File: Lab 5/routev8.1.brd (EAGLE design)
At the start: 100 x 80 mm, 48 parts, among them J1 FTDI_DEVICE, M1 WIRELESS-NRF24L01, U2 GY-521MPU6050, U3 ATMEGA328P_TQFP

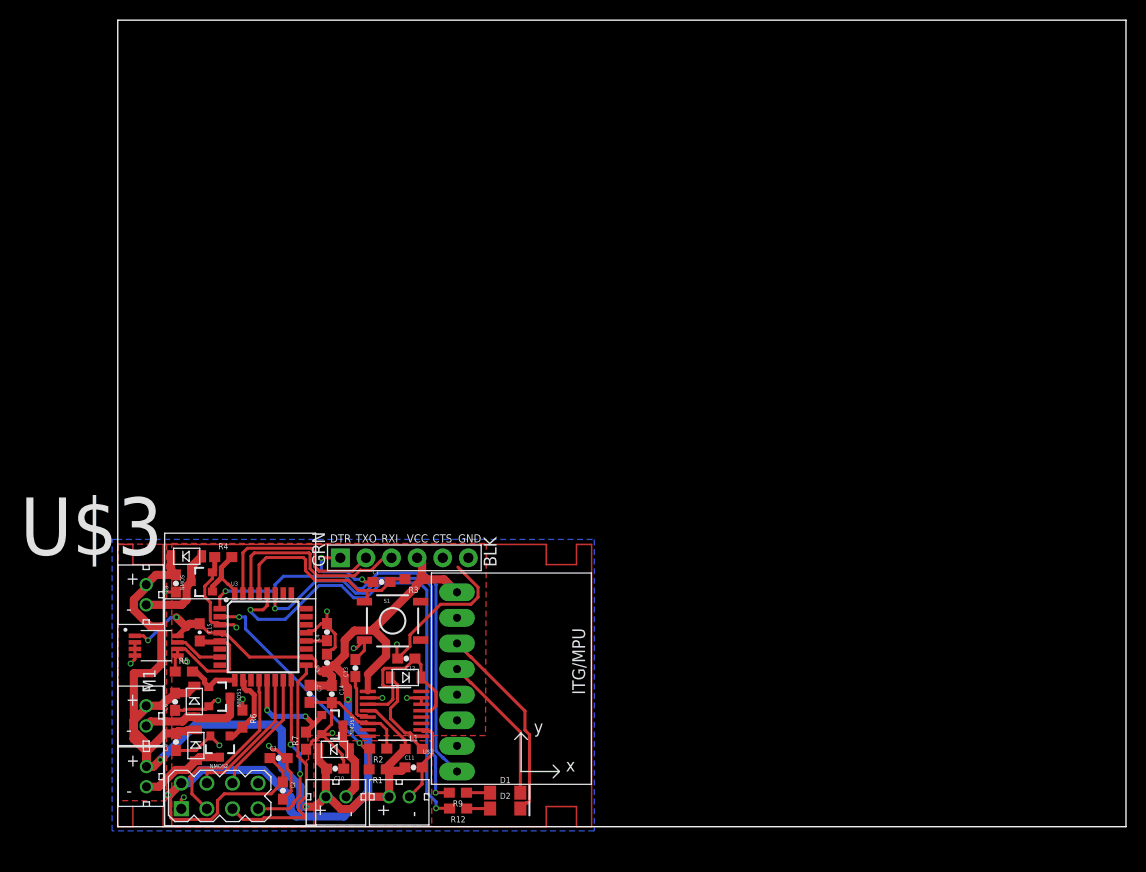
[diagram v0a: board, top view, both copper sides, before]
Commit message: We need a redesign guys
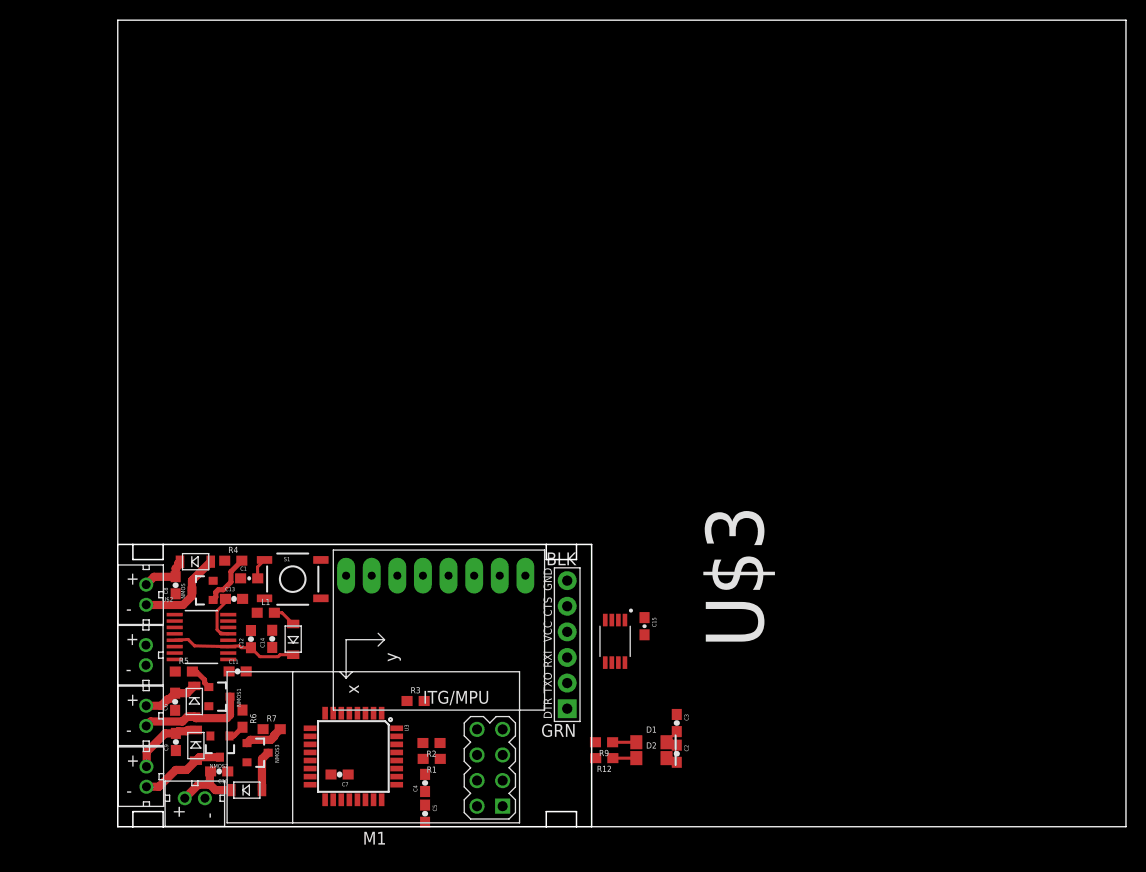
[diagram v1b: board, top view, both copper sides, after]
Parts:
- removed J1: FTDI_DEVICE, quad:FTDI_DEVICE_SIDE
- added J2: FTDI_DEVICE, quad:FTDI_DEVICE_SIDE
- C1: device SparkFun-Passives:0603-CAP -> SparkFun-Capacitors:0603-CAP
- R3: value 1k -> 10k
- moved U$3 45.5 mm to (49.3, 18.4), turned to 270 degrees
- moved C15 44.1 mm to (52.2, 19.9)
- moved C3 39.6 mm to (55.4, 10.3), turned to 270 degrees
- moved C2 39.2 mm to (55.4, 7.24)
- moved MOTOR3 23.5 mm to (2.79, 17.0), turned to 0 degrees
- moved U$2 20.6 mm to (8.30, 18.8), turned to 0 degrees
- moved U$1 20.3 mm to (7.65, 2.83)
- moved L1 19.9 mm to (14.7, 21.2)
- moved C11 19.9 mm to (11.9, 15.4)
- moved C4 17.8 mm to (30.5, 4.34)
- moved C5 17.8 mm to (30.5, 1.30), turned to 270 degrees
- moved C12 15.5 mm to (13.2, 18.6), turned to 90 degrees
- moved D1 15.3 mm to (52.9, 8.38)
- moved D2 15.3 mm to (52.9, 6.80)
- moved R12 15.3 mm to (48.3, 6.80)
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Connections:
- removed net N$13: C1.1, J1.P$1
- new net N$12: C1.1, J2.P$1
- net FTDI-RX: now also J2.P$3; no longer J1.P$3
- net FTDI-TX: now also J2.P$2; no longer J1.P$2
- net GND: now also J2.P$6; no longer J1.P$6
- net RESET: now also R3.1; no longer R3.2
- net VCC: now also J2.P$4, R3.2; no longer J1.P$4, R3.1
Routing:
- net N$11: track 163.0 -> 0.00 mm
- net VCC: track 113.2 -> 0.00 mm, vias 4 -> 0
- net GND: track 111.0 -> 0.00 mm, vias 15 -> 0
- net BATTERY+: track 99.2 -> 24.5 mm, vias 2 -> 0
- net N$10: track 47.2 -> 0.00 mm, vias 2 -> 0
- net IMU-INT: track 45.0 -> 0.00 mm, vias 1 -> 0
- net N$8: track 41.6 -> 0.00 mm, vias 2 -> 0
- net RF-SCK: track 24.0 -> 0.00 mm
- net MEASURE_PIN: track 23.1 -> 0.00 mm, vias 2 -> 0
- net FTDI-RX: track 20.3 -> 0.00 mm
- net IMU-SCL: track 19.8 -> 0.00 mm
- net RESET: track 21.3 -> 2.12 mm
- net FTDI-TX: track 18.8 -> 0.00 mm
- net RF-CE: track 17.7 -> 0.00 mm
- net RF-MISO: track 16.7 -> 0.00 mm, vias 2 -> 0
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- removed copper zone on layer 1, net BATTERY_+
- removed copper zone on layer 16, net GND
- removed copper zone on layer 1, net S$1
- removed copper zone on layer 1, net S$2
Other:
- outline, holes or cut-outs redrawn
